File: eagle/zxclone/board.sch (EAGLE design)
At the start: 21 parts, among them IC15 74LS151N, IC17 74LS151N, IC2 74LS86N, IC3 74LS74N, IC4 74LS04N

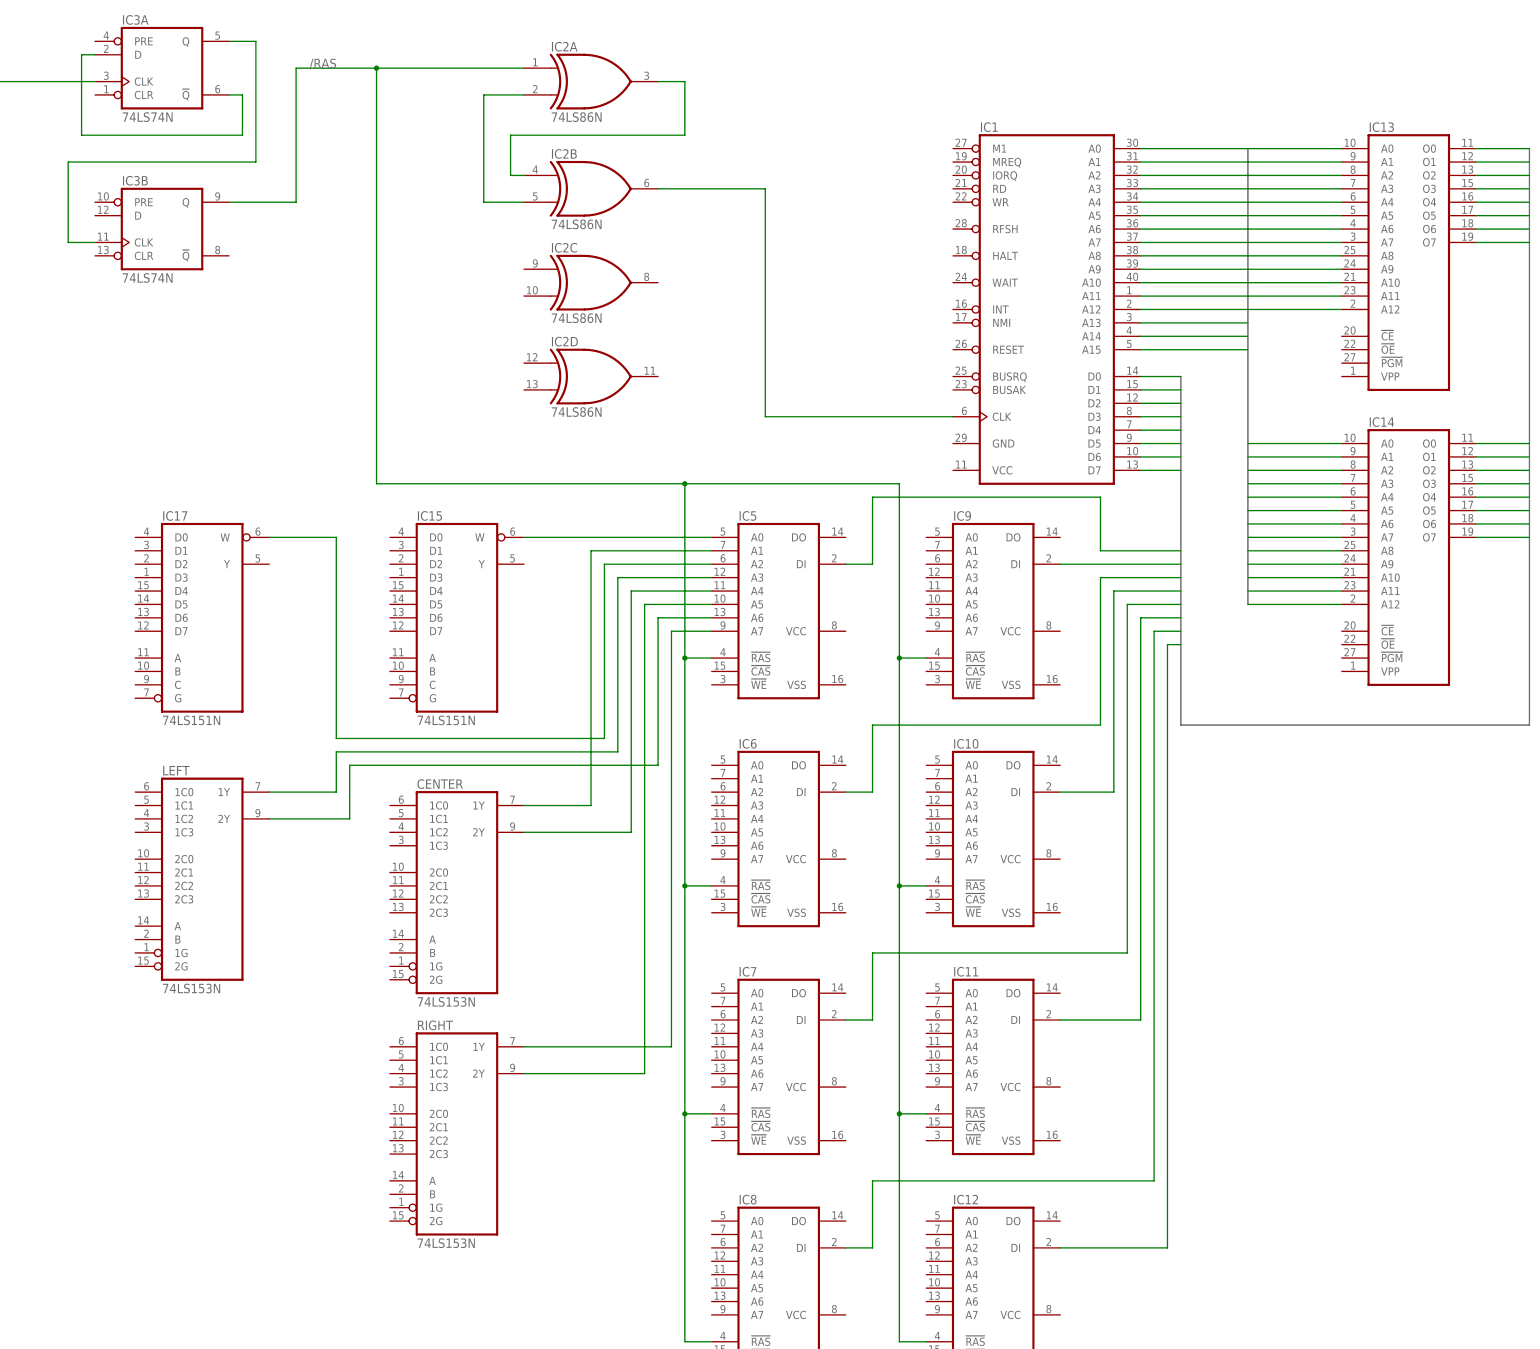
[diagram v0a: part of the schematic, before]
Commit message: sdsda
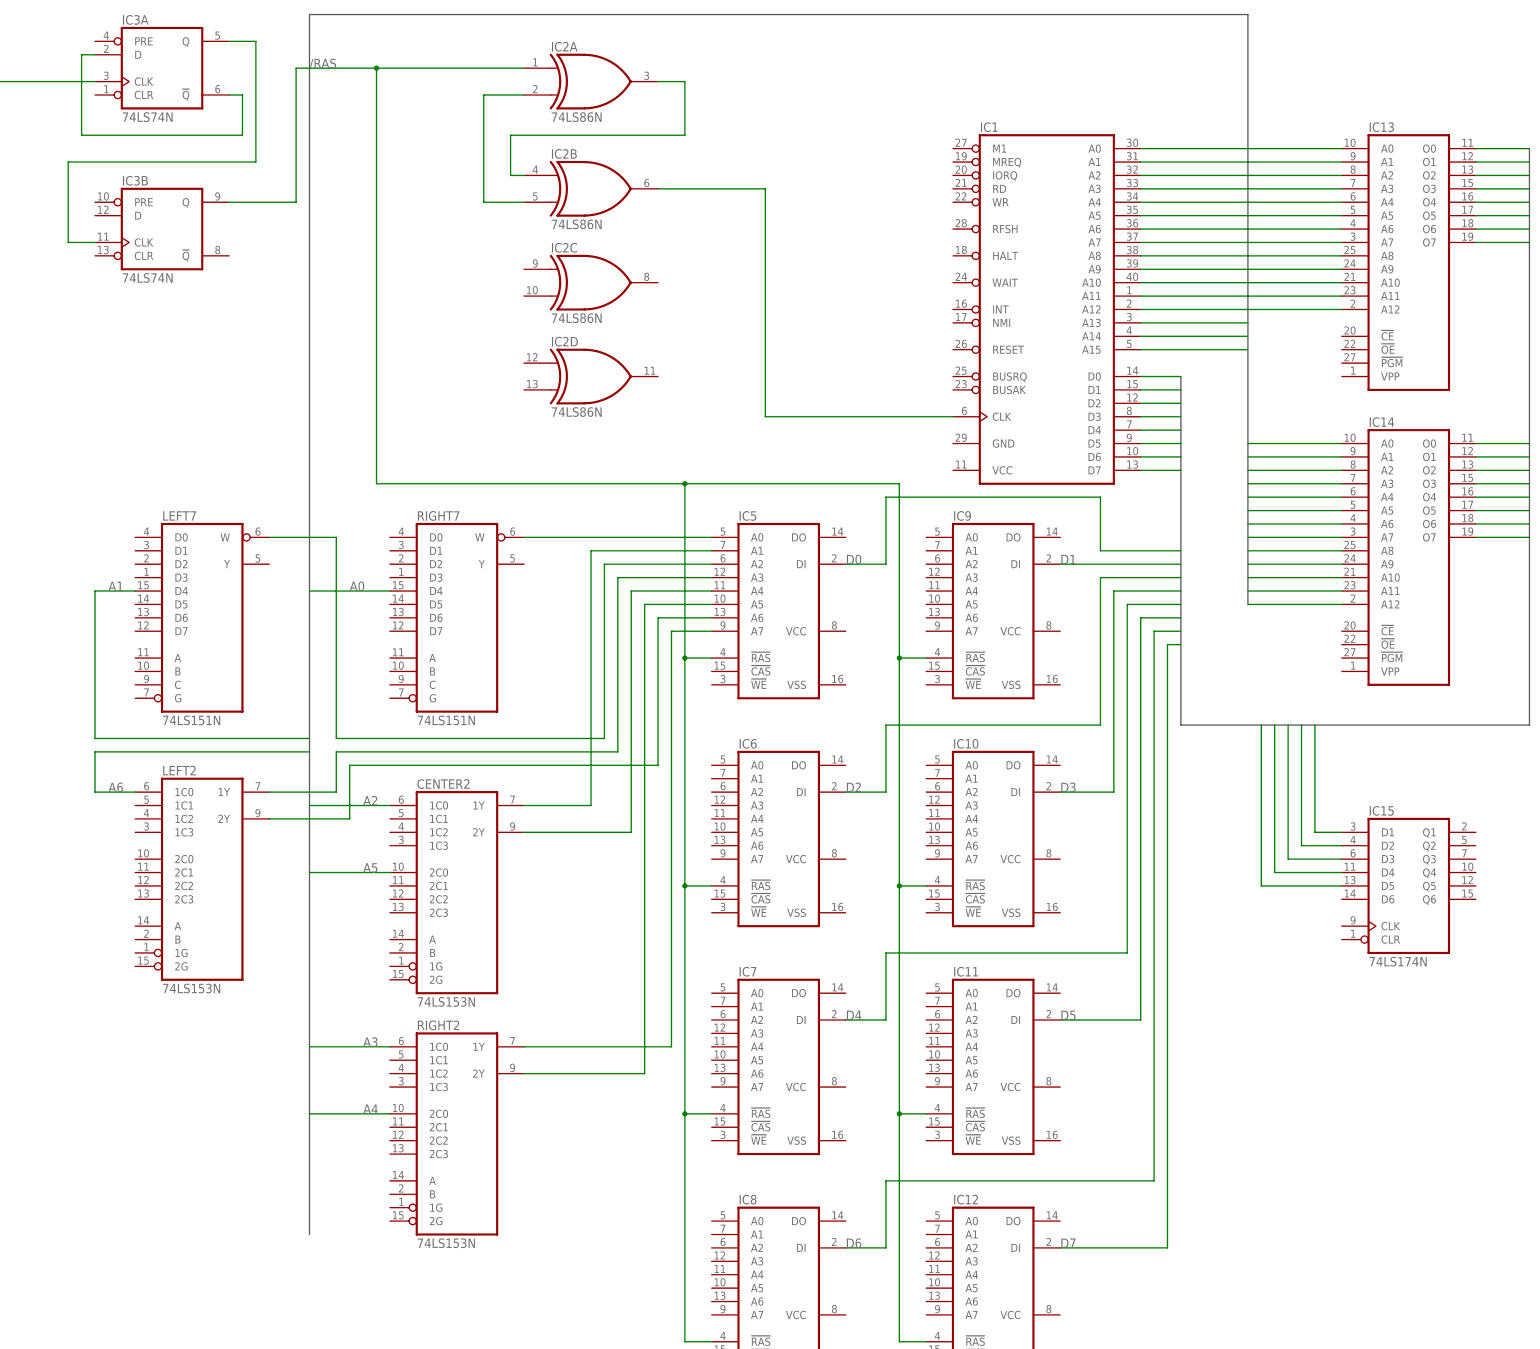
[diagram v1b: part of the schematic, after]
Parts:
- added RIGHT7: 74LS151N, 74xx-us:74LS151N
- IC15: value 74LS151N -> 74LS174N; device 74xx-us:74LS151N -> 74xx-us:74LS174N
- renumbered CENTER to CENTER2, IC17 to LEFT7, LEFT to LEFT2, RIGHT to RIGHT2
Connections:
- net A0: now also RIGHT7A.D4
- net A1: now also LEFT7A.D4
- net A2: now also CENTER2A.1C0
- net A3: now also RIGHT2A.1C0
- net A4: now also RIGHT2A.2C0
- net A5: now also CENTER2A.2C0
- net A6: now also LEFT2A.1C0
- net D0: now also IC15A.D1
- net D1: now also IC15A.D2
- net D2: now also IC15A.D3
- net D3: now also IC15A.D4
- net D4: now also IC15A.D5
- net N$9: now also RIGHT7A.W; no longer IC15A.W
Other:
- moved on the sheet: IC15

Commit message: more
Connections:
- removed net N$10: CENTER2A.1Y, IC5.A1
- removed net N$11: IC5.A2, LEFT7A.W
- removed net N$12: IC5.A3, LEFT2A.1Y
- removed net N$13: CENTER2A.2Y, IC5.A4
- removed net N$14: IC5.A5, RIGHT2A.2Y
- removed net N$15: IC5.A6, LEFT2A.2Y
- removed net N$16: IC5.A7, RIGHT2A.1Y
- removed net N$9: IC5.A0, RIGHT7A.W
- new net MA0: IC10.A0, IC11.A0, IC12.A0, IC5.A0, IC6.A0, IC7.A0, IC8.A0, IC9.A0, RIGHT7A.W
- new net MA1: CENTER2A.1Y, IC10.A1, IC11.A1, IC12.A1, IC5.A1, IC6.A1, IC7.A1, IC8.A1, IC9.A1
- new net MA2: IC10.A2, IC11.A2, IC12.A2, IC5.A2, IC6.A2, IC7.A2, IC8.A2, IC9.A2, LEFT7A.W
- new net MA3: IC10.A3, IC11.A3, IC12.A3, IC5.A3, IC6.A3, IC7.A3, IC8.A3, IC9.A3, LEFT2A.1Y
- new net MA4: CENTER2A.2Y, IC10.A4, IC11.A4, IC12.A4, IC5.A4, IC6.A4, IC7.A4, IC8.A4, IC9.A4
- new net MA5: IC10.A5, IC11.A5, IC12.A5, IC5.A5, IC6.A5, IC7.A5, IC8.A5, IC9.A5, RIGHT2A.2Y
- new net MA6: IC10.A6, IC11.A6, IC12.A6, IC5.A6, IC6.A6, IC7.A6, IC8.A6, IC9.A6, LEFT2A.2Y
- new net MA7: IC10.A7, IC11.A7, IC12.A7, IC5.A7, IC6.A7, IC7.A7, IC8.A7, IC9.A7, RIGHT2A.1Y
- net A10: now also CENTER2A.1C1
- net A11: now also RIGHT2A.1C1
- net A12: now also RIGHT2A.2C1
- net A13: now also CENTER2A.2C1
- net A14: now also LEFT2A.1C1
- net A15: now also LEFT2A.2C1
- net A7: now also LEFT2A.2C0
- net A8: now also RIGHT7A.D5
- net A9: now also LEFT7A.D5
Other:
- moved on the sheet: CENTER2, IC10, IC11, IC12, IC15, IC5, IC6, IC7, IC8, IC9, LEFT2, LEFT7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

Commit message: shit
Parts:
- added IC16: 74LS02N, 74xx-us:74LS02N
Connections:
- new net GND: IC1.GND, IC10.VSS, IC11.VSS, IC12.VSS, IC5.VSS, IC6.VSS, IC7.VSS, IC8.VSS, IC9.VSS
- new net N$9: IC10.!CAS, IC11.!CAS, IC12.!CAS, IC16A.O, IC5.!CAS, IC6.!CAS, IC7.!CAS, IC8.!CAS, IC9.!CAS
- new net VCC: IC1.VCC, IC10.VCC, IC11.VCC, IC12.VCC, IC5.VCC, IC6.VCC, IC7.VCC, IC8.VCC, IC9.VCC
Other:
- moved on the sheet: IC2A, IC2B, IC2C, IC2D
